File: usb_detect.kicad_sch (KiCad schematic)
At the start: 3 parts

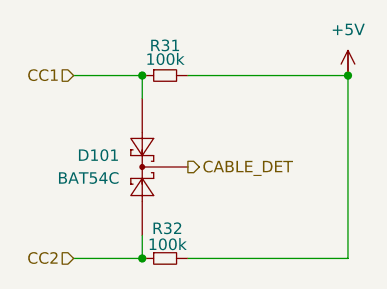
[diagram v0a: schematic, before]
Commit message: update ERC
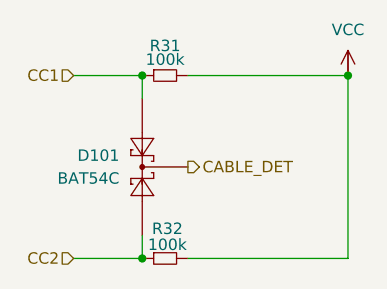
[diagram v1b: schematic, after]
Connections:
- net +5V renamed VCC
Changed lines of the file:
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@@
 	)
 	(symbol
-		(lib_id "G-Love:+5V")
+		(lib_id "G-Love:VCC")
 		(at 118.11 77.47 0)
 		(unit 1)
@@
 			)
 		)
-		(property "Value" "+5V"
+		(property "Value" "VCC"
 			(at 118.11 73.66 0)
 			(show_name no)

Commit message: pcb v06 good
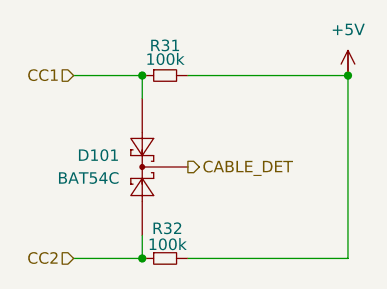
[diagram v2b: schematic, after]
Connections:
- net VCC renamed +5V
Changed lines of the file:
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@@
 	)
 	(symbol
-		(lib_id "G-Love:VCC")
+		(lib_id "G-Love:+5V")
 		(at 118.11 77.47 0)
 		(unit 1)
@@
 			)
 		)
-		(property "Value" "VCC"
+		(property "Value" "+5V"
 			(at 118.11 73.66 0)
 			(show_name no)
